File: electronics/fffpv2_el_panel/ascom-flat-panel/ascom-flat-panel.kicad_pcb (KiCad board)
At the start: 2 copper layers, 56 x 32 mm, 14 parts, among them J1 Servo, J2 JST-XH LED, Q1 IRLZ34N, Q2 IRLZ34N, U1 XIAO-SAMD21-DIP

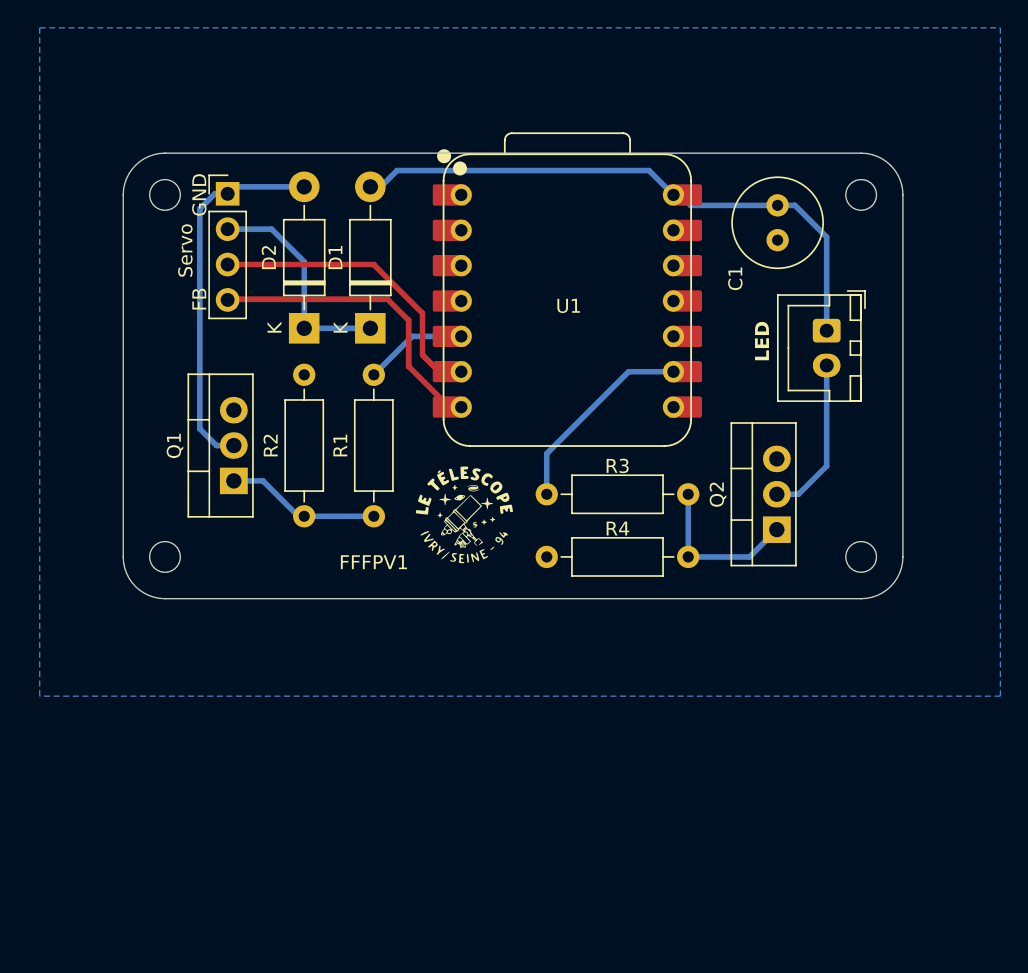
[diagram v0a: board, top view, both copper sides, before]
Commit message: [electronics] - intialisation PCB v2. Gros travail de routage en perspective :D
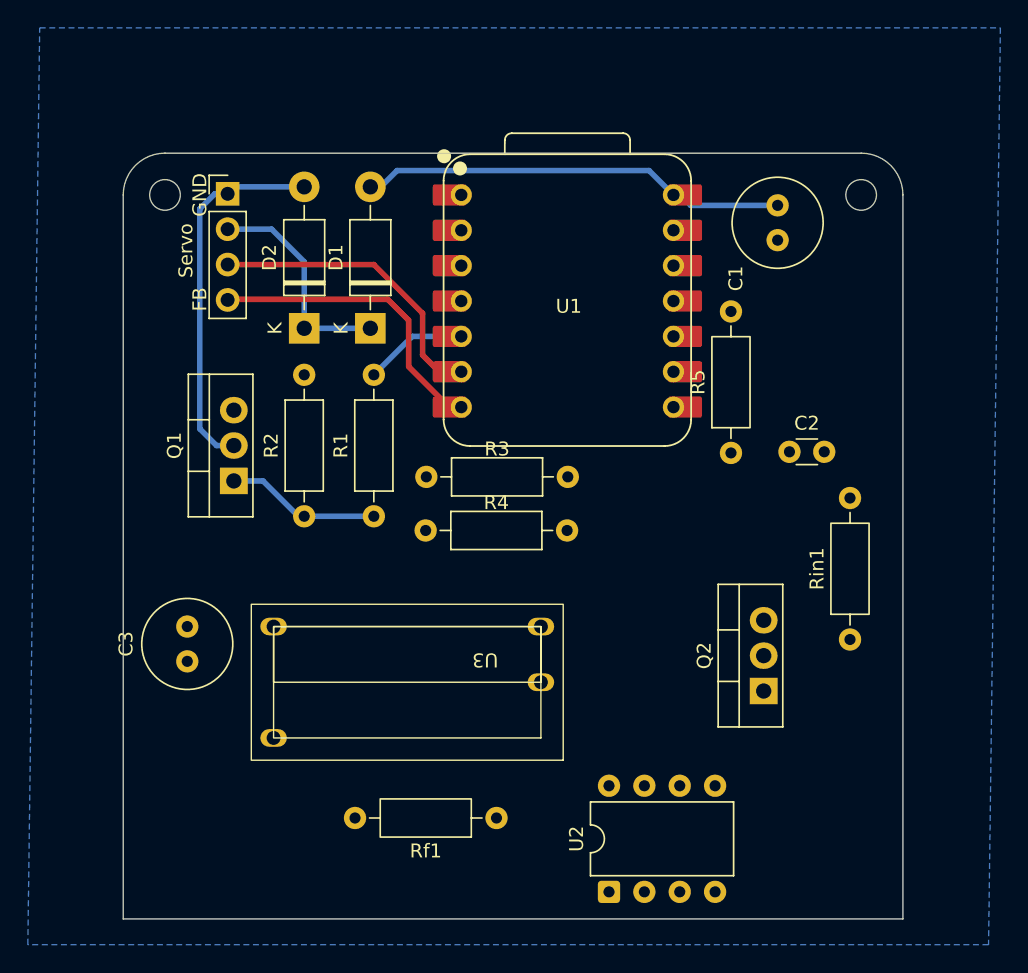
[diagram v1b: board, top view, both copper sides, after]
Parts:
- removed the G*** at (120.5, 96.0)
- removed J2: JST-XH LED, Connector_JST:JST_XH_B2B-XH-A_1x02_P2.50mm_Vertical
- added C2: 22nF, Capacitor_THT:C_Disc_D3.0mm_W1.6mm_P2.50mm, F.Cu at (143.8, 91.5)
- added C3: 10µF, Capacitor_THT:C_Radial_D6.3mm_H11.0mm_P2.50mm, F.Cu at (100.6, 106.5)
- added R5: 1M, Resistor_THT:R_Axial_DIN0207_L6.3mm_D2.5mm_P10.16mm_Horizontal, F.Cu at (139.7, 91.5)
- added Rf1: 82k, Resistor_THT:R_Axial_DIN0207_L6.3mm_D2.5mm_P10.16mm_Horizontal, F.Cu at (122.8, 117.8)
- added Rin1: 38kΩ, Resistor_THT:R_Axial_DIN0207_L6.3mm_D2.5mm_P10.16mm_Horizontal, F.Cu at (148.2, 104.9)
- added U2: TLC272, Package_DIP:DIP-8_W7.62mm, F.Cu at (130.9, 123.1)
- added U3: ~, CustomFootprints:DFR052 DC regulator, F.Cu at (116.4, 108.1)
- moved Q2 11.6 mm to (142.0, 108.6)
- moved R4 8.91 mm to (127.9, 97.1)
- moved R3 8.74 mm to (117.8, 93.2)
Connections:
- Q2 pad 2: Net-(J2-Pin_2) -> EL PANEL CONTROL CIRCUIT
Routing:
- net LED_STRIP_POWER_CONTROL: track 14.5 -> 0.00 mm
- net Net-(Q2-G): track 11.7 -> 0.00 mm
- net Net-(J2-Pin_2): track 11.6 -> 0.00 mm
- net +5V: track 41.2 -> 30.0 mm
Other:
- board size 56 x 32 mm -> 56 x 55 mm
- board text removed: "LED"
